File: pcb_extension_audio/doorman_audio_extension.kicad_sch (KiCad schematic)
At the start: 37 parts, among them J1 Audio Out, J4 Extension Board Connector, J5 Audio In, U1 ES8388

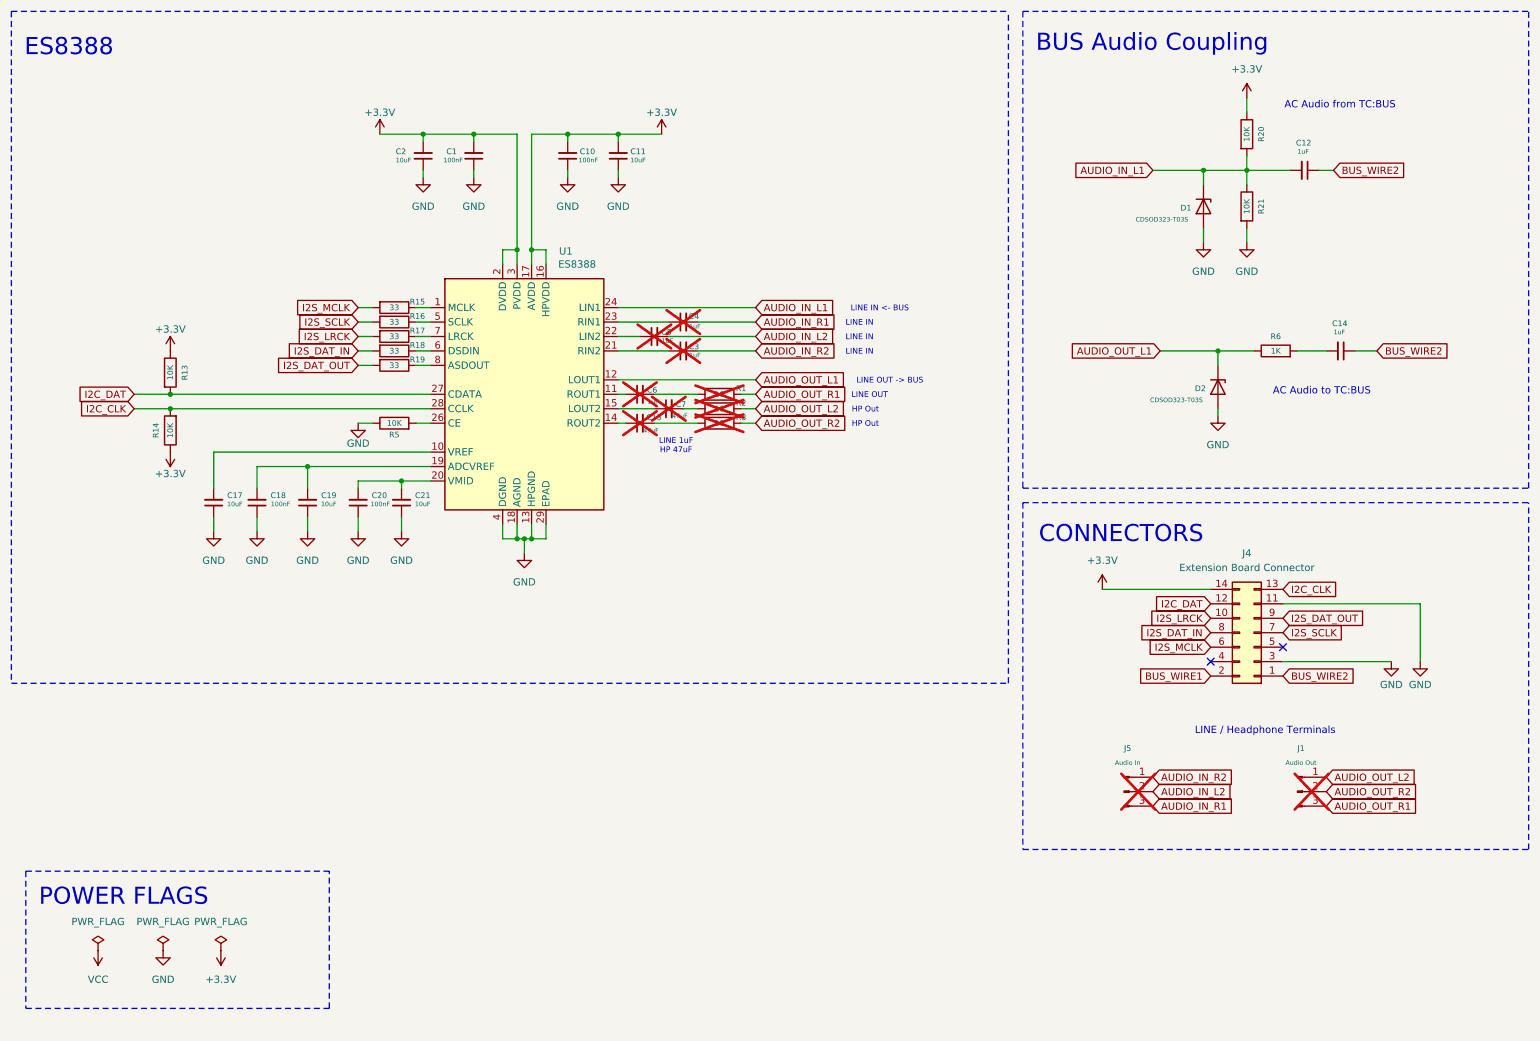
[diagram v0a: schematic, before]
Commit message: WIP
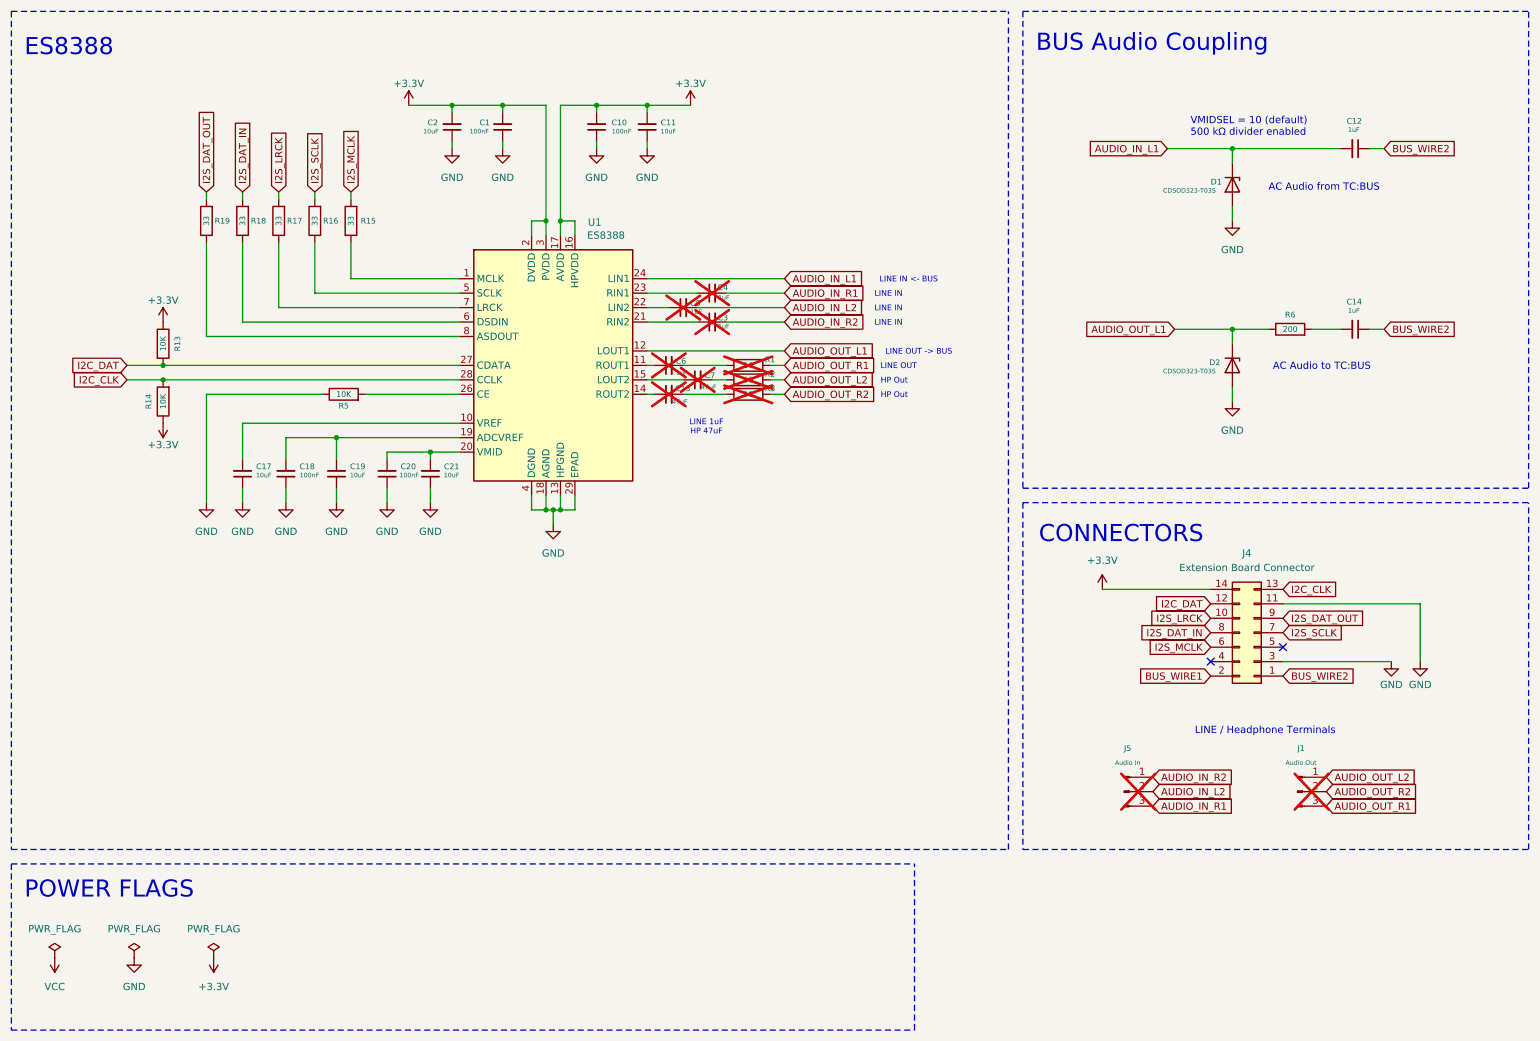
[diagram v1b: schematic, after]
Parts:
- removed R20, R21: 10K, Resistor_SMD:R_0603_1608Metric, symbol Device:R
- R6: value 1K -> 200
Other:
- note added: "VMIDSEL = 10 (default) 500 kΩ divider enabled"
- moved on the sheet: C1, C10, C11, C12, C13, C14, C17, C18, C19, C2, C20, C21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
